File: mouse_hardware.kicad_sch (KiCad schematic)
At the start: 16 parts, among them U1 TPS73601DBV, U2 TPS73601DBV

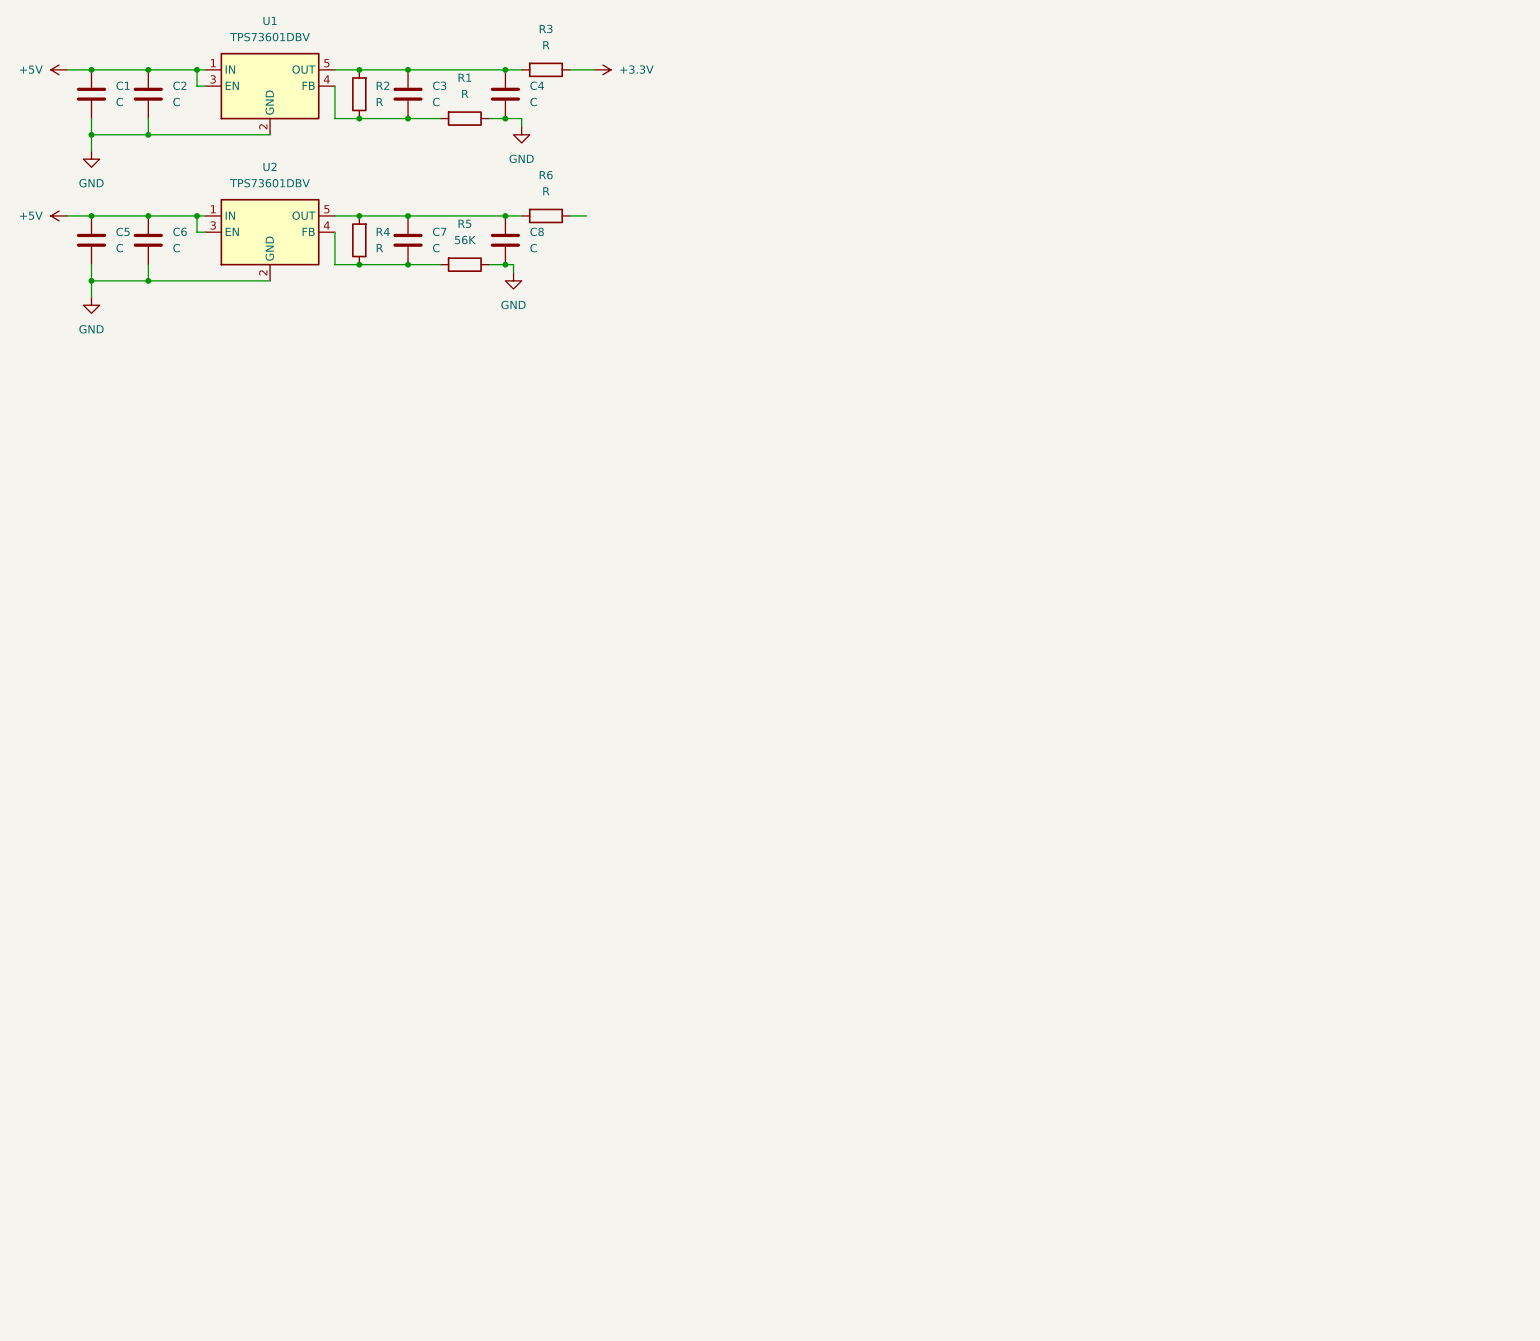
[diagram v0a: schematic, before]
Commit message: Start designing pcb
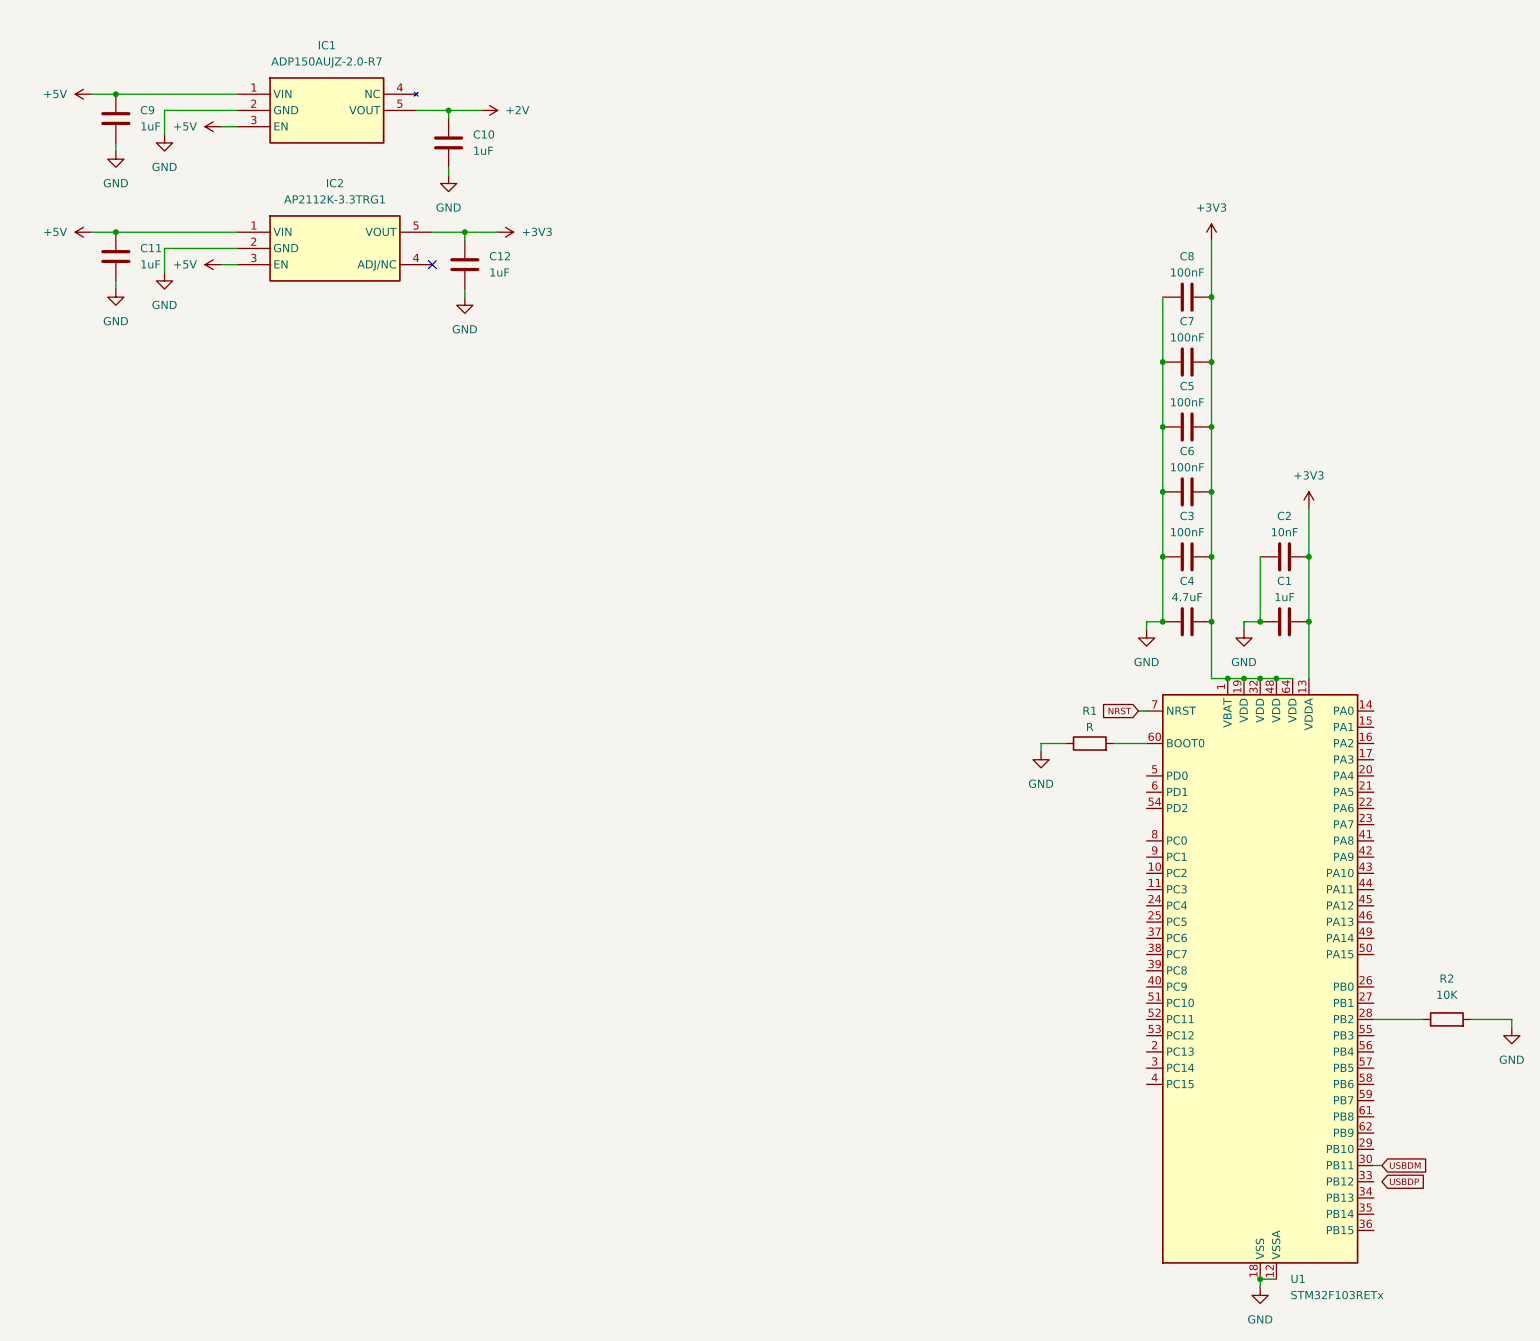
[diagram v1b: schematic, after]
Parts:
- removed R3, R4, R6: R, symbol Device:R
- removed R5: 56K, symbol Device:R
- removed U1, U2: TPS73601DBV, Package_TO_SOT_SMD:SOT-23-5, symbol Regulator_Linear:TPS73601DBV
- added C10, C11, C12, C9: 1uF, symbol Device:C
- added IC1: ADP150AUJZ-2.0-R7, SOT95P280X100-5N, symbol ADP150AUJZ:ADP150AUJZ-2.0-R7
- added IC2: AP2112K-3.3TRG1, SOT95P282X130-5N, symbol AP2112K-3:AP2112K-3.3TRG1
- added U1: STM32F103RETx, Package_QFP:LQFP-64_10x10mm_P0.5mm, symbol MCU_ST_STM32F1:STM32F103RETx
- C1: value C -> 1uF
- C2: value C -> 10nF
- C3, C5, C6, C7, C8: value C -> 100nF
- C4: value C -> 4.7uF
- R2: value R -> 10K
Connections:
- net +5V: now also C11.2, C9.2, IC1.1 (VIN), IC1.3 (EN), IC2.1 (VIN), IC2.3 (EN); no longer C1.1, C2.1, C5.1, C6.1
- net GND: now also C3.2, C7.2, R2.2, C10.1, C11.1, C12.1, C9.1, IC1.2 (GND), IC2.2 (GND), U1.12 (VSSA), U1.18 (VSS), U1.31 (VSS), U1.47 (VSS), U1.63 (VSS)
- net +3V3: now reaches C7.1, C8.1
- net +3V3: now also C1.1, C2.1, C3.1, C4.1, C5.1, C6.1, C12.2, IC2.5 (VOUT), U1.1 (VBAT), U1.13 (VDDA), U1.19 (VDD), U1.32 (VDD), U1.48 (VDD), U1.64 (VDD)
- new net: R2.1, U1.28 (PB2)
- new net: R1.2, U1.60 (BOOT0)
- new net +2V: C10.2, IC1.5 (VOUT)
- new net NRST: U1.7 (NRST)
- new net USBDM: U1.30 (PB11)
- no-connect marks 0 -> 1
